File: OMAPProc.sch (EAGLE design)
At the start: 41 parts, among them IC1 MIC5335-SPYMT, IC2 MIC5335-MGYMT, IC3 TXS0108ERGY

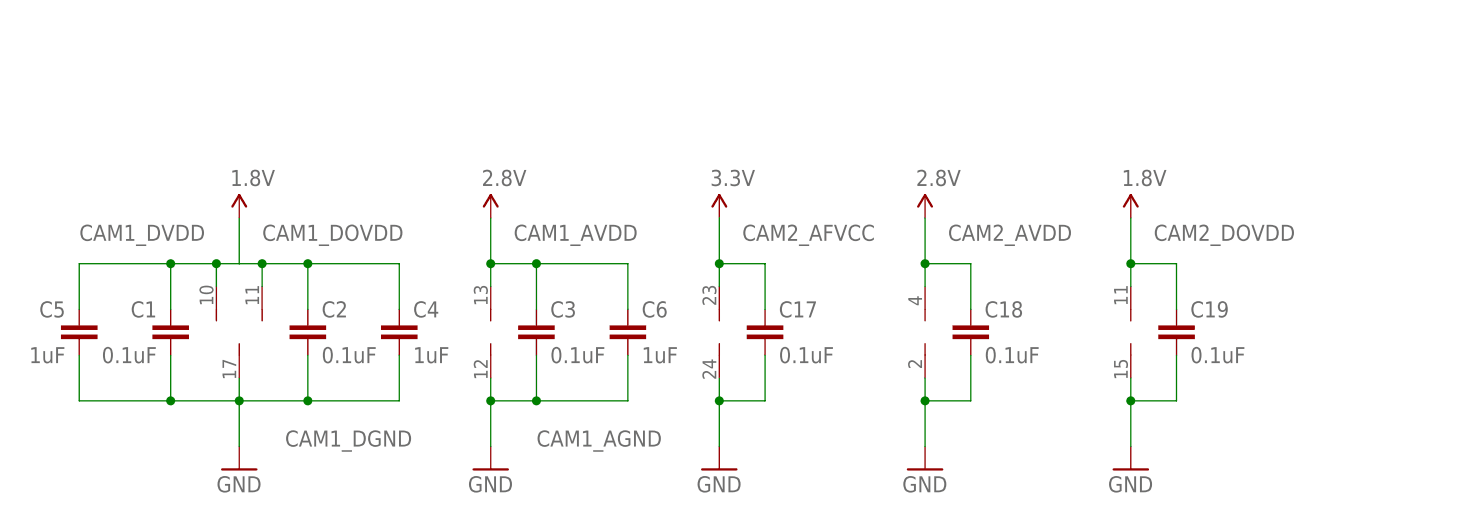
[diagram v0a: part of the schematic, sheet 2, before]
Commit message: Near-final placement, partial route
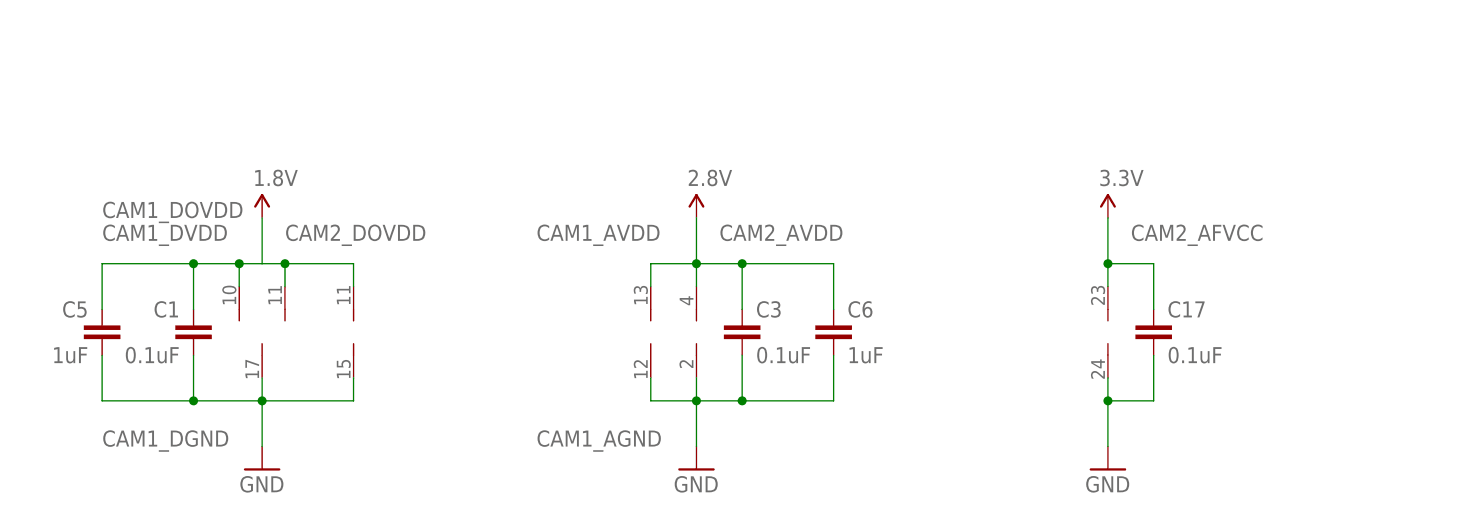
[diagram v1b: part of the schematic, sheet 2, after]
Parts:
- removed C18, C19, C2: 0.1uF, biomimetic:CAP0402-CAP
- removed C4: 1uF, biomimetic:CAP0402-CAP
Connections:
- net 1.8V: no longer C19.1, C2.1, C4.1
- net 2.8V: no longer C18.1
- net GND: no longer C18.2, C19.2, C2.2, C4.2
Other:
- moved on the sheet: C1, C17, C3, C5, C6, CAM1_AGND, CAM1_AVDD, CAM1_DGND, CAM1_DOVDD, CAM1_DVDD, CAM2_AFVCC, CAM2_AVDD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
